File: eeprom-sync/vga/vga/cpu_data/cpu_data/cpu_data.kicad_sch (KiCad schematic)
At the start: 34 parts, among them J1 Conn_02x06_Odd_Even, J10 Conn_01x03_Female, J11 Conn_01x02_Female, J12 Conn_02x05_Odd_Even, J2 Conn_01x02_Female, J3 Conn_01x04_Female, J4 Conn_01x15_Female, J5 Conn_01x15_Female, J6 Conn_02x08_Odd_Even, J7 Conn_01x02_Female, J8 Conn_01x02_Female, J9 Conn_01x08_Female, Q1 Q_PNP_BEC, U1 GAL22V10, U2 74HC14, U3 74LS02, U4 IDT7205L12JG, U5 74LS573

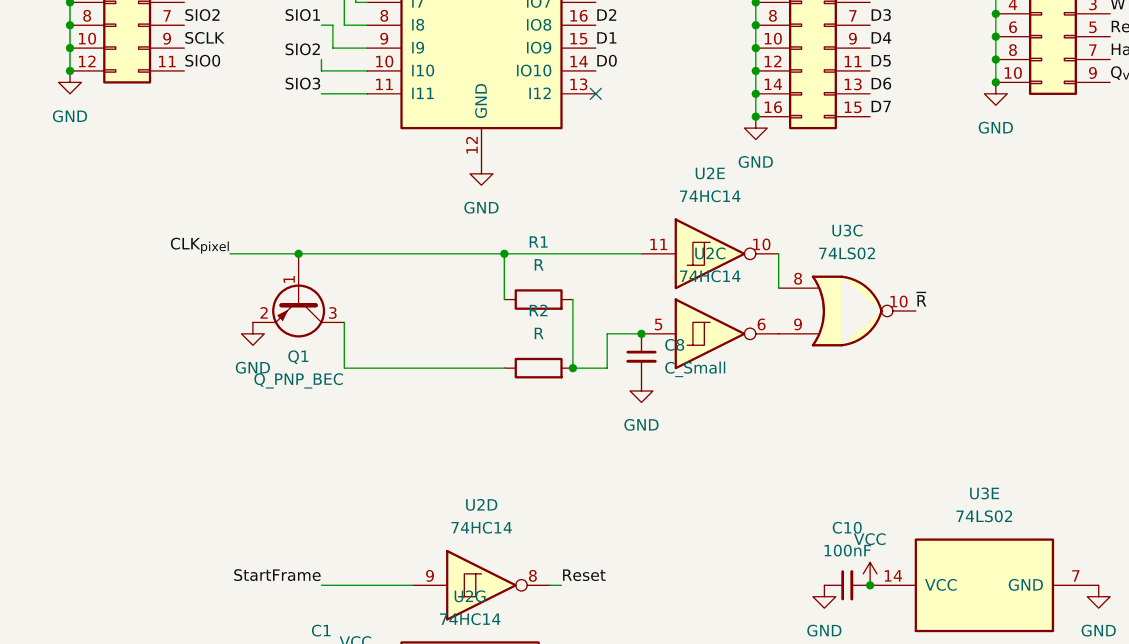
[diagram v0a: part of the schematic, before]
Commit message: finalized form of pcb and schematic
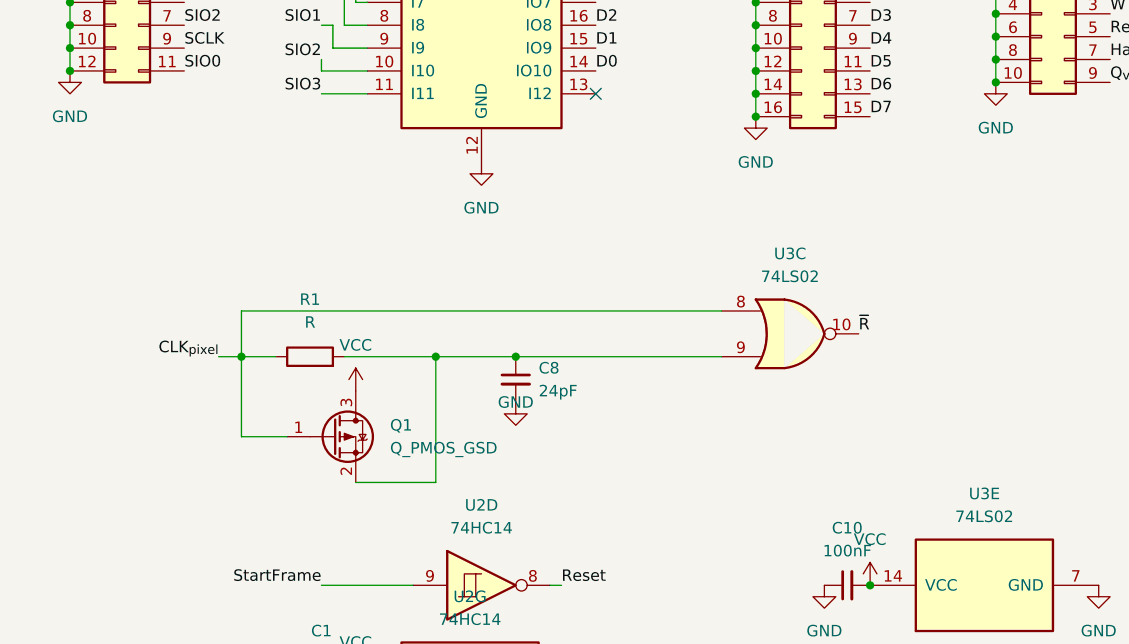
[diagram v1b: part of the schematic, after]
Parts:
- removed Q1: Q_PNP_BEC, Package_TO_SOT_SMD:SOT-323_SC-70_Handsoldering, symbol Device:Q_PNP_BEC
- removed R2: R, Resistor_SMD:R_0805_2012Metric_Pad1.20x1.40mm_HandSolder, symbol Device:R
- removed unit 5 of U2
- removed unit 3 of U2
- added Q1: Q_PMOS_GSD, Package_TO_SOT_SMD:SOT-323_SC-70_Handsoldering, symbol Device:Q_PMOS_GSD
- C8: value C_Small -> 24pF; Product (none) -> https://www.mouser.com/ProductDetail/KEMET/C0603C240G1HACTU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
- U3: Product (none) -> https://www.mouser.com/ProductDetail/Texas-Instruments/SN74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
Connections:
- net CLK_{pixel}: now also U3.8, Q1.1 (G)
- net VCC: now also Q1.3 (D)
- net at C8.1, R1.2: now also U3.9, Q1.2 (S)
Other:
- moved on the sheet: C8, U3C
